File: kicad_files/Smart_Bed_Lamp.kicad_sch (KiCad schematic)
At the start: 0 parts

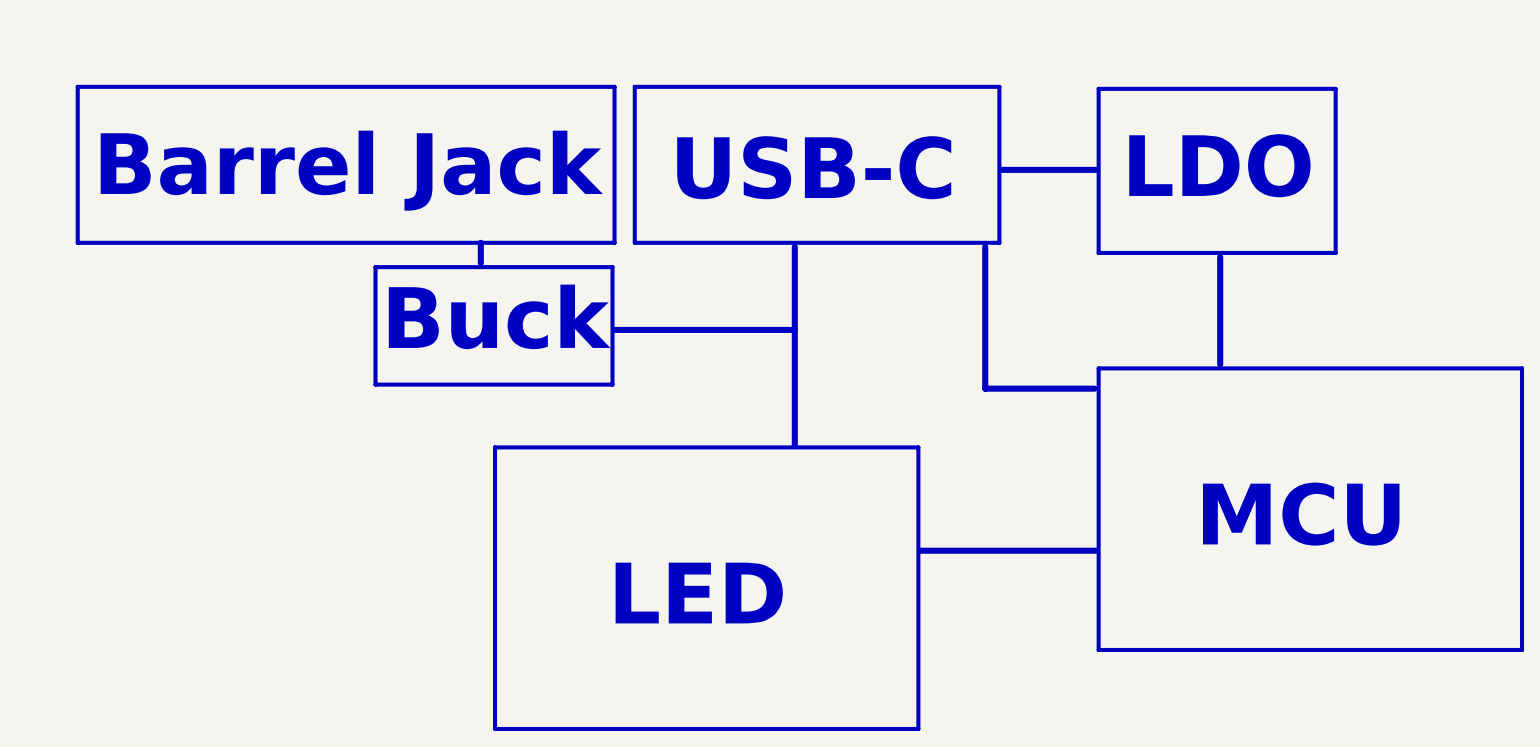
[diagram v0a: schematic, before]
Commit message: Add files via upload
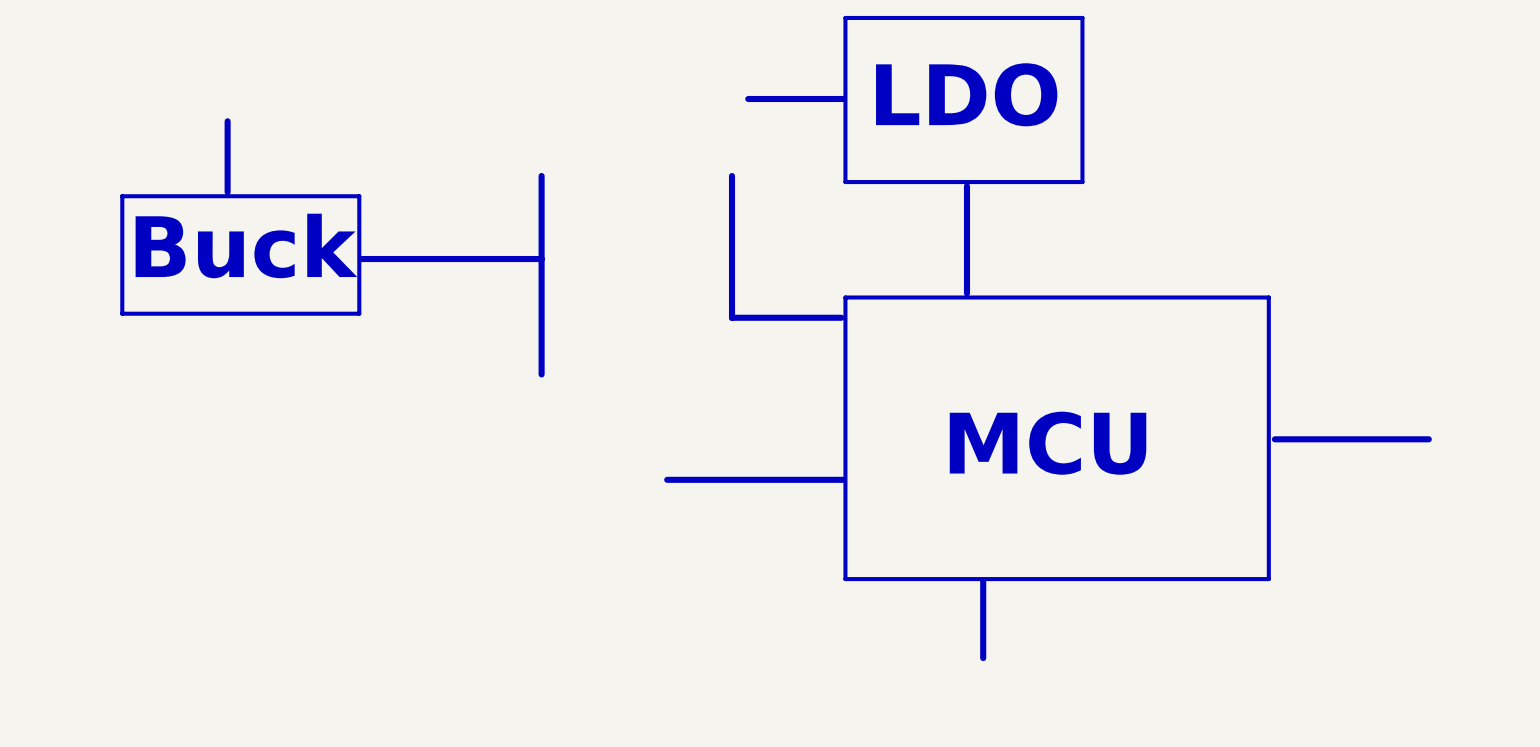
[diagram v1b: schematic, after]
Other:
- note removed: "Barrel Jack"
- note removed: "LED"
- note removed: "USB-C"
